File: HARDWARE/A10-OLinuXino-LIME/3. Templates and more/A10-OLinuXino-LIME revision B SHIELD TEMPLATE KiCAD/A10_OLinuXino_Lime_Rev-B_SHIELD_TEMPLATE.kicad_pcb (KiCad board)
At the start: 2 copper layers, 53.2 x 59.6 mm, 5 parts

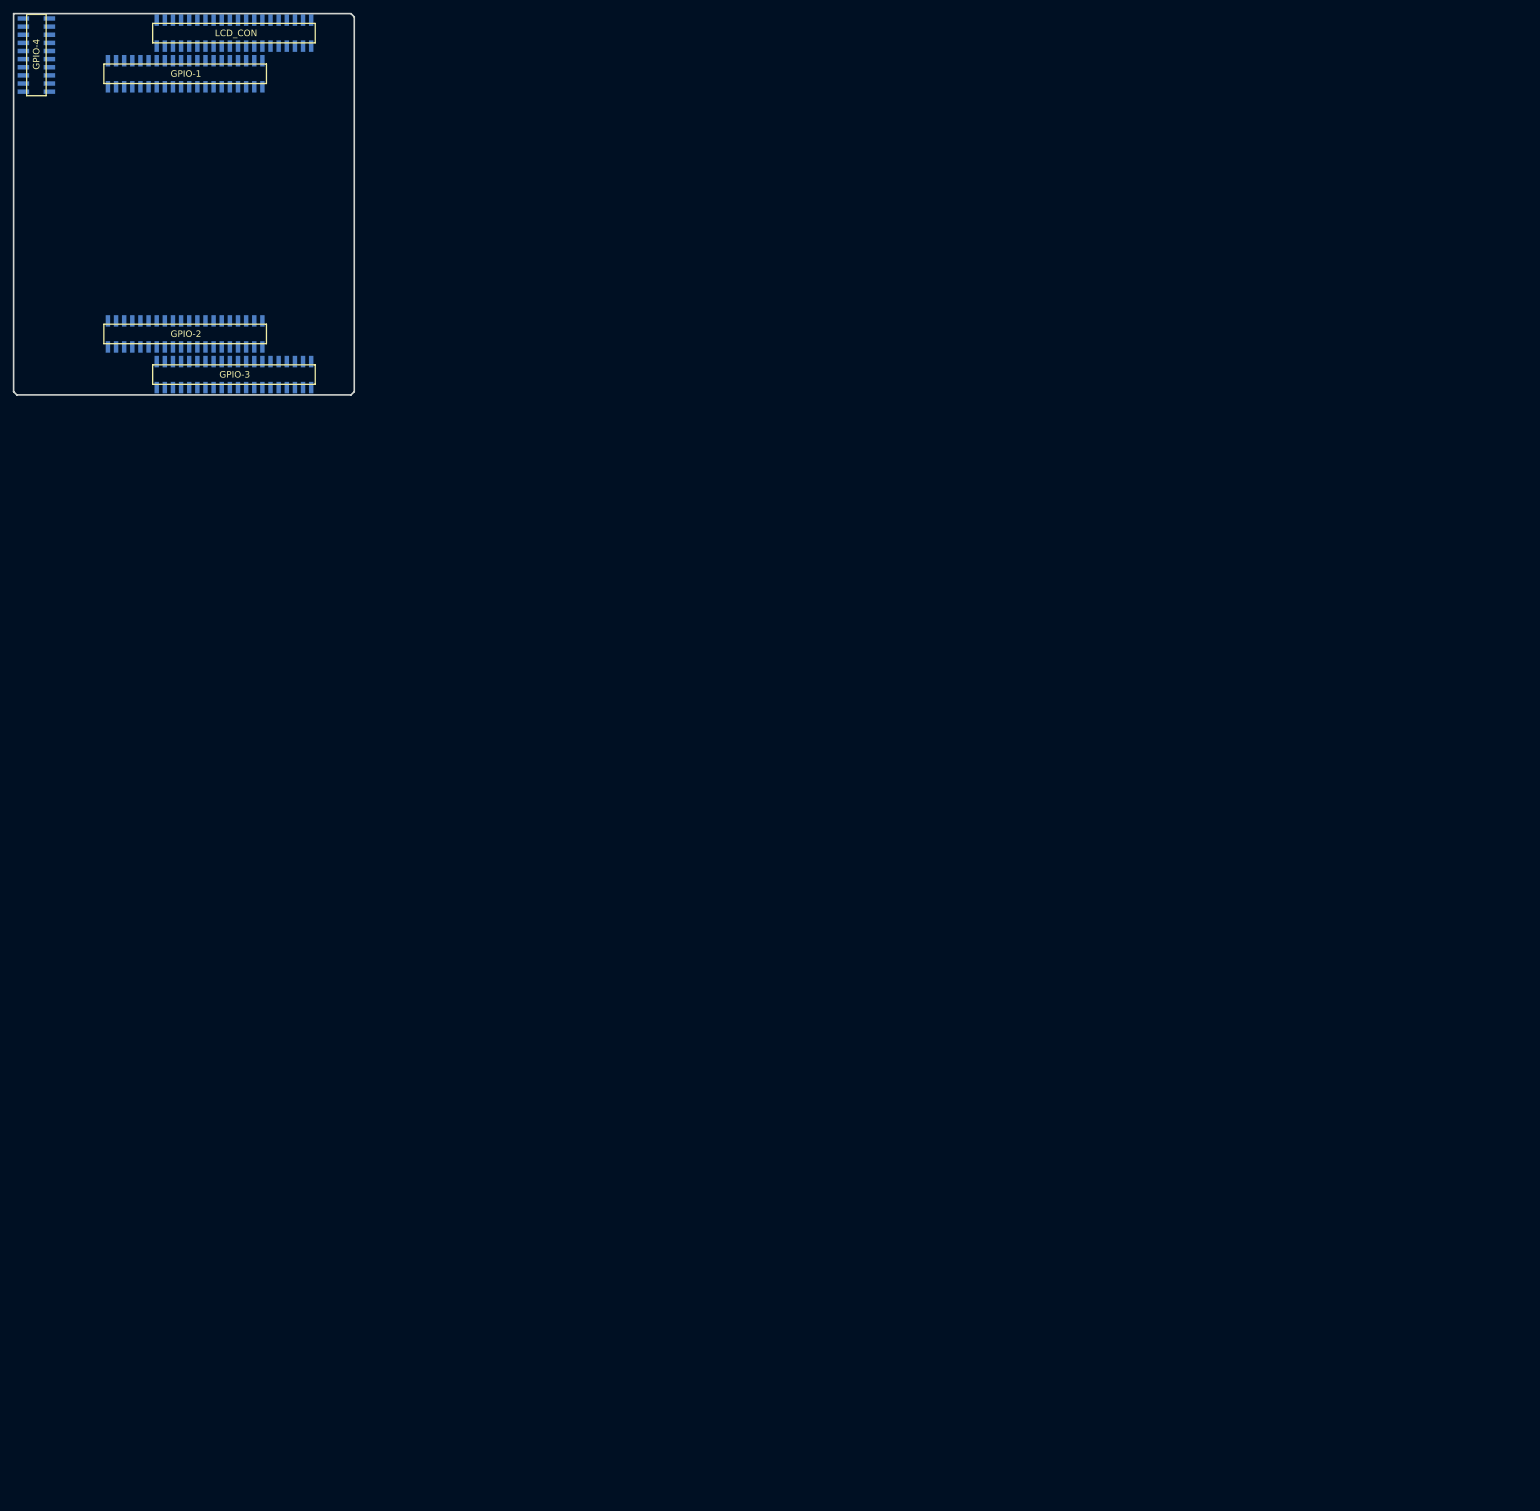
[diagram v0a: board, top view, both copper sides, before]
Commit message: Update
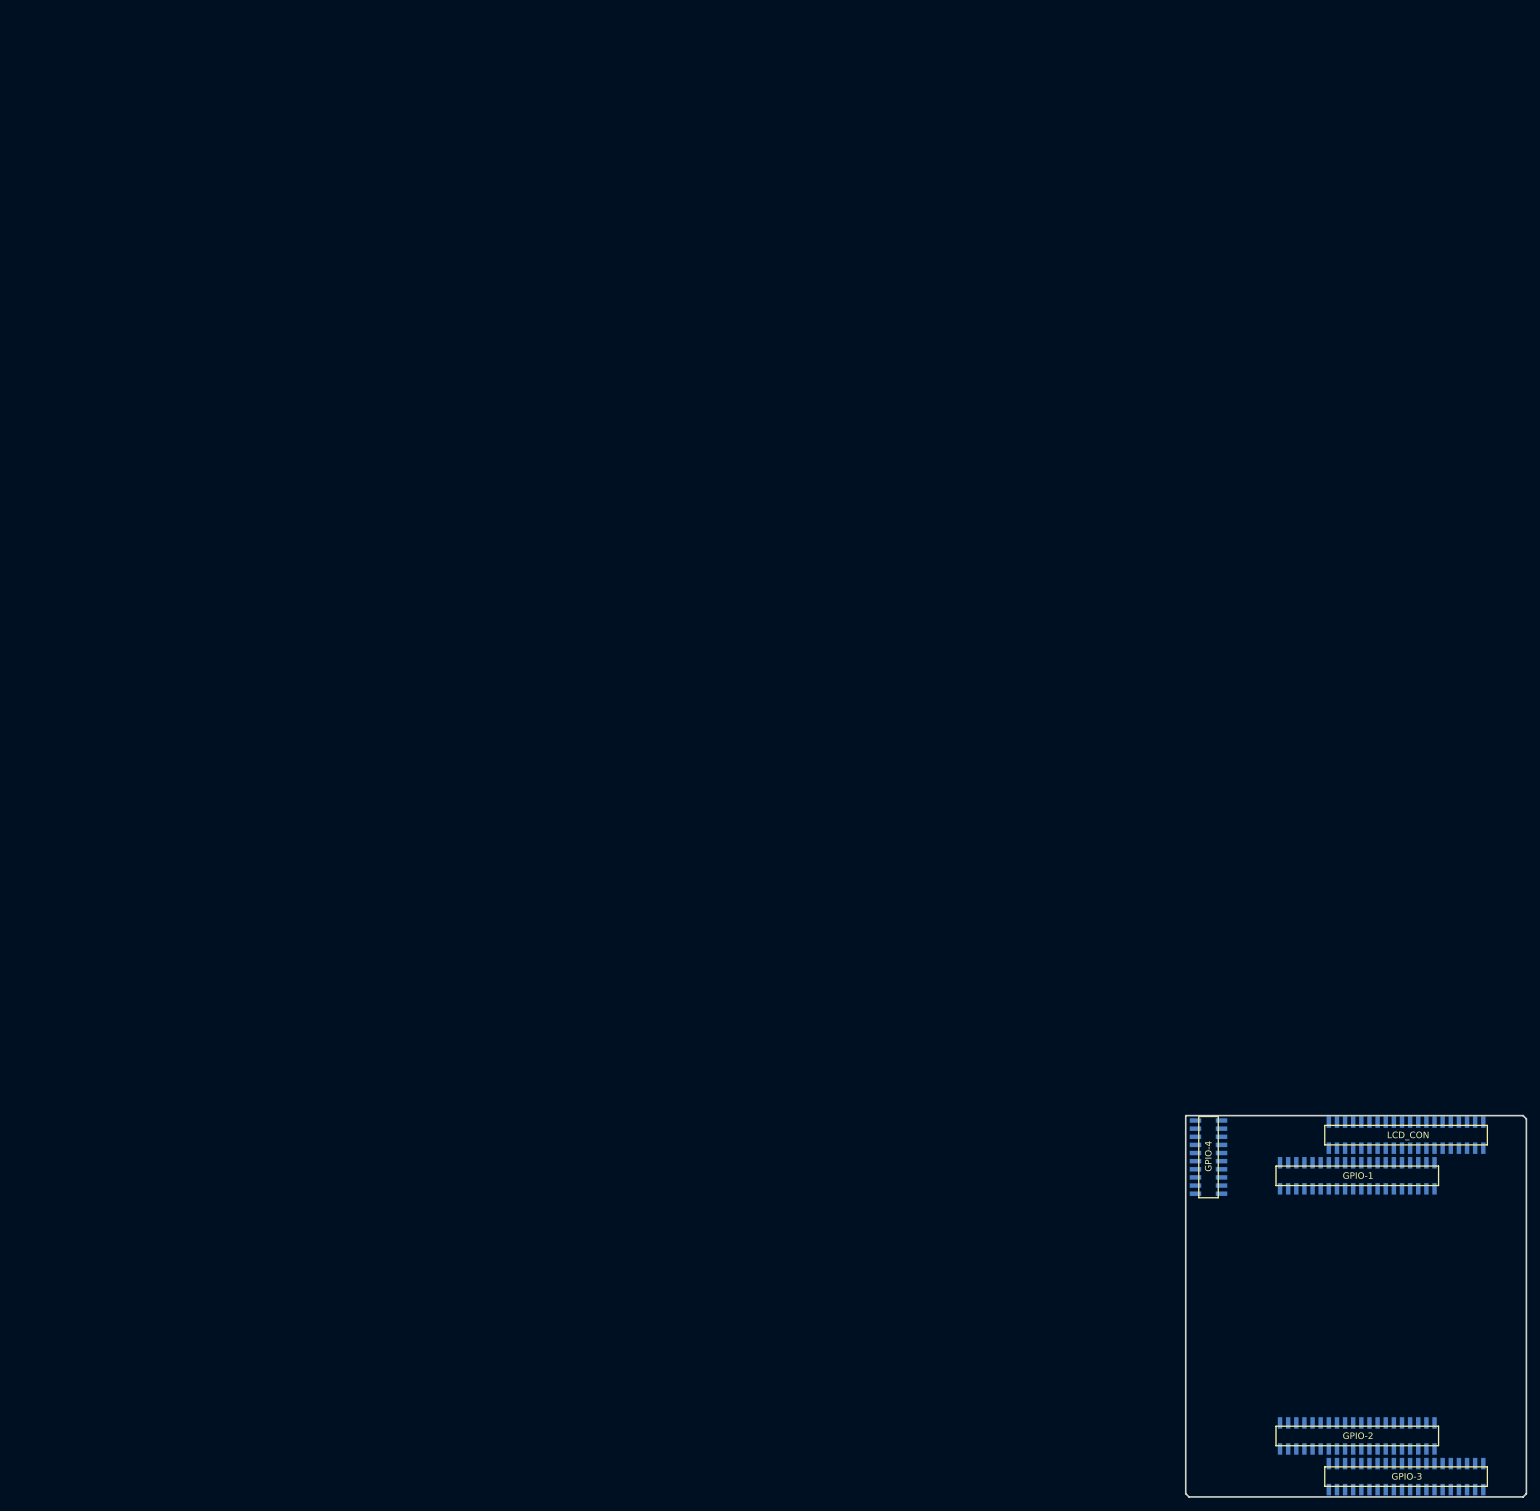
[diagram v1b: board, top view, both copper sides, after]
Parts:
- moved GPIO-1 251.3 mm to (183.3, 151.8)
- moved GPIO-2 251.3 mm to (183.3, 192.4)
- moved LCD_CON1 251.3 mm to (190.9, 145.4)
- moved GPIO-4 251.3 mm to (160.0, 148.8)
- moved GPIO-3 251.3 mm to (190.9, 198.8)
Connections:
- GPIO-1 pad 10: (no net) -> /MICIN1
- GPIO-1 pad 11: (no net) -> /TS1_DVLD/CSI1_VSYNC/SDC1_D1/PG3
- GPIO-1 pad 12: (no net) -> /VMIC
- GPIO-1 pad 13: (no net) -> /TS1_D0/CSI1_D0/SDC1_D2/CSI0_D8/PG4
- GPIO-1 pad 14: (no net) -> /HPOUTL
- GPIO-1 pad 15: (no net) -> /TS1_D1/CSI1_D1/SDC1_D3/CSI0_D9/PG5
- GPIO-1 pad 16: (no net) -> /HPCOM/HPCOMFB
- GPIO-1 pad 17: (no net) -> /TS1_D2/CSI1_D2/UART3_TX/CSI0_D10/PG6
- GPIO-1 pad 18: (no net) -> /HPOUTR
- GPIO-1 pad 19: (no net) -> /TS1_D3/CSI1_D3/UART3_RX/CSI0_D11/PG7
- GPIO-1 pad 20: (no net) -> /TVOUT0/VGA-G
- GPIO-1 pad 21: (no net) -> /TS1_D4/CSI1_D4/UART3_RTS/CSI0_D12/PG8
- GPIO-1 pad 22: (no net) -> /TVOUT1/VGA-B
- GPIO-1 pad 23: (no net) -> /TS1_D5/CSI1_D5/UART3_CTS/CSI0_D13/PG9
- GPIO-1 pad 24: (no net) -> /TVOUT2/VGA-R
- GPIO-1 pad 25: (no net) -> /TS1_D6/CSI1_D6/UART4_TX/CSI0_D14/PG10
- GPIO-1 pad 26: (no net) -> /UART0_RX/IR1_RX/PB23
- GPIO-1 pad 27: (no net) -> /TS1_D7/CSI1_D7/UART4_RX/CSI0_D15/PG11
- GPIO-1 pad 28: (no net) -> /UART0_TX/IR1_TX/PB22
- GPIO-1 pad 29: (no net) -> /NCE1/PC3/SATA-PWR-EN
- GPIO-1 pad 3: +3.3V -> +3V3
- GPIO-1 pad 30: (no net) -> /TWI2_SDA/PB21
- GPIO-1 pad 31: (no net) -> /NCE3/PC18
- GPIO-1 pad 32: (no net) -> /TWI2_SCK/PB20
- GPIO-1 pad 33: (no net) -> /NCE4/SPI2_CS0/PC19
- GPIO-1 pad 34: (no net) -> /TWI1_SDA/PB19
- GPIO-1 pad 35: (no net) -> /NCE5/SPI2_CLK/PC20
- GPIO-1 pad 36: (no net) -> /TWI1_SCK/PB18
- GPIO-1 pad 37: (no net) -> /NCE6/SPI2_MOSI/PC21
- GPIO-1 pad 38: (no net) -> /NDQS/PC24
- GPIO-1 pad 39: (no net) -> /NCE7/SPI2_MISO/PC22
- GPIO-1 pad 4: (no net) -> GNDPWR
- GPIO-1 pad 40: (no net) -> /SPI0_CS0/PC23
- GPIO-1 pad 5: (no net) -> /TS1_CLK/CSI1_PCLK/SDC1_CMD/PG0
- GPIO-1 pad 6: (no net) -> /LRADC0
- GPIO-1 pad 7: (no net) -> /TS1_ERR/CSI1_MLCK/SDC1_CLK/PG1
- GPIO-1 pad 8: (no net) -> /LRADC1
- GPIO-1 pad 9: (no net) -> /TS1_SYNC/CSI1_HSYNC/SDC1_D0/PG2
- GPIO-2 pad 10: (no net) -> /TS0_SYNC/CSI0_HSYNC/PE2
- GPIO-2 pad 11: (no net) -> /GPS_SIGN/PI1
- GPIO-2 pad 12: (no net) -> /TS0_DVLD/CSI0_VSYNC/PE3
- GPIO-2 pad 13: (no net) -> /GPS_MAG/PI2
- GPIO-2 pad 14: (no net) -> /TS0_D0/CSI0_D0/PE4
- GPIO-2 pad 15: (no net) -> /PWM1/PI3
- GPIO-2 pad 16: (no net) -> /TS0_D1/CSI0_D1/PE5
- GPIO-2 pad 17: (no net) -> /SDC3_CMD/PI4
- GPIO-2 pad 18: (no net) -> /TS0_D2/CSI0_D2/PE6
- GPIO-2 pad 19: (no net) -> /SDC3_CLK/PI5
- GPIO-2 pad 20: (no net) -> /TS0_D3/CSI0_D3/PE7
- GPIO-2 pad 21: (no net) -> /SDC3_D0/PI6
- GPIO-2 pad 22: (no net) -> /TS0_D4/CSI0_D4/PE8
- GPIO-2 pad 23: (no net) -> /SDC3_D1/PI7
- GPIO-2 pad 24: (no net) -> /TS0_D5/CSI0_D5/PE9
- GPIO-2 pad 25: (no net) -> /SDC3_D2/PI8
- GPIO-2 pad 26: (no net) -> /TS0_D6/CSI0_D6/PE10
- GPIO-2 pad 27: (no net) -> /SDC3_D3/PI9
- GPIO-2 pad 28: (no net) -> /TS0_D7/CSI0_D7/PE11
- GPIO-2 pad 29: (no net) -> /SPI0_CS0/UART5_TX/EINT22/PI10
- GPIO-2 pad 3: +3.3V -> +3V3
- GPIO-2 pad 30: (no net) -> /HSDA/UART7_RX/PS2_SDA0/PI21
- GPIO-2 pad 31: (no net) -> /SPI0_CLK/UART5_RX/EINT23/PI11
- GPIO-2 pad 32: (no net) -> /HSCL/UART7_TX/PS2_SCK0/PI20
- GPIO-2 pad 33: (no net) -> /SPI0_MOSI/UART6_TX/EINT24/PI12
- GPIO-2 pad 34: (no net) -> /EINT31/SPI1_MISO/UART2_RX/PI19
- GPIO-2 pad 35: (no net) -> /SPI0_MISO/UART6_RX/EINT25/PI13
- GPIO-2 pad 36: (no net) -> /EINT30/SPI1_MOSI/UART2_TX/PI18
- GPIO-2 pad 37: (no net) -> /PS2_SCK1/TCLKIN0/EINT26/SPI0_CS1/PI14
- GPIO-2 pad 38: (no net) -> /EINT29/SPI1_CLK/UART2_CTS/PI17
- GPIO-2 pad 39: (no net) -> /PS2_SDA1/TCLKIN1/EINT27/SPI1_CS1/PI15
- GPIO-2 pad 4: (no net) -> /LDO3_2.8V/VCC_CSI0
- GPIO-2 pad 40: (no net) -> /EINT28/SPI1_CS0/UART2_RTS/PI16
- GPIO-2 pad 5: (no net) -> /TWI0_SCK/PB0
- GPIO-2 pad 6: (no net) -> /TS0_CLK/CSI0_PCLK/PE0
- GPIO-2 pad 7: (no net) -> /TWI0_SDA/PB1
- GPIO-2 pad 8: (no net) -> /TS0_ERR/CSI0_MCLK/PE1
- GPIO-2 pad 9: (no net) -> /GPS_CLK/PI0
- GPIO-3 pad 10: (no net) -> /I2S_MCLK/AC97_MCLK/PB5
- GPIO-3 pad 11: (no net) -> /LCD1_D9/ATAD5/KP_IN1/MS_D1/EINT9/CSI1_D9/PH9
- GPIO-3 pad 12: (no net) -> /I2S_BCLK/AC97_BCLK/PB6
- GPIO-3 pad 13: (no net) -> /LCD1_D10/ATAD6/KP_IN2/MS_D2/EINT10/CSI1_D10/PH10
- GPIO-3 pad 14: (no net) -> /I2S_LRCK/AC97_SYNC/PB7
- GPIO-3 pad 15: (no net) -> /LCD1_D11/ATAD7/KP_IN3/MS_D3/EINT11/CSI1_D11/PH11
- GPIO-3 pad 16: (no net) -> /I2S_DO0/AC97_DO/PB8/SATA-PWR-EN
- GPIO-3 pad 17: (no net) -> /LCD1_D12/ATAD8/PS2_SCK1/EINT12/CSI1_D12/PH12
- GPIO-3 pad 18: (no net) -> /I2S_DO2/PB10
- GPIO-3 pad 19: (no net) -> /LCD1_D13/ATAD9/PS2_SDA1/SMC_RST/EINT13/CSI1_D13/PH13
- GPIO-3 pad 20: (no net) -> /I2S_DO3/PB11
- GPIO-3 pad 21: (no net) -> /LCD1_D14/ATAD10/KP_IN4/SMC_VPPEN/EINT14/CSI1_D14/PH14
- GPIO-3 pad 22: (no net) -> /I2S_DI/AC97_DI/SPDIF_DI/PB12
- GPIO-3 pad 23: (no net) -> /LCD1_D15/ATAD11/KP_IN5/SMC_VPPPP/EINT15/CSI1_D15/PH15
- GPIO-3 pad 24: (no net) -> /SPI2_CS1/SPDIF_DO/PB13
- GPIO-3 pad 25: (no net) -> /LCD1_D16/ATAD12/KP_IN6/SMC_DET/EINT16/CSI1_D16/PH16
- GPIO-3 pad 26: (no net) -> /JTAG_MS0/SPI2_CS0/PB14
- GPIO-3 pad 27: (no net) -> /LCD1_D17/ATAD13/KP_IN7/SMC_VCCEN/EINT17/CSI1_D17/PH17
- GPIO-3 pad 28: (no net) -> /JTAG_CK0/SPI2_CLK/PB15
- GPIO-3 pad 29: (no net) -> /LCD1_D18/ATAD14/KP_OUT0/SMC_SLK/EINT18/CSI1_D18/PH18
- GPIO-3 pad 3: (no net) -> +3V3
- GPIO-3 pad 30: (no net) -> /JTAG_DO0/SPI2_MOSI/PB16
- GPIO-3 pad 31: (no net) -> /LCD1_D19/ATAD15/KP_OUT1/SMC_SDA/EINT19/CSI1_D19/PH19
- GPIO-3 pad 32: (no net) -> /JTAG_DI0/SPI2_MISO/PB17
- GPIO-3 pad 33: (no net) -> /LCD1_D20/ATAOE/CAN_TX/EINT20/CSI1_D20/PH20
- GPIO-3 pad 34: (no net) -> /LCD1_CLK/ATACS1/KP_OUT4/SDC1_D0/CSI1_PCLK/PH24
- GPIO-3 pad 35: (no net) -> /LCD1_D21/ATADREQ/CAN_RX/EINT21/CSI1_D21/PH21
- GPIO-3 pad 36: (no net) -> /LCD1_DE/ATAIORDY/KP_OUT5/SDC1_D1/CSI1_FIELD/PH25
- GPIO-3 pad 37: (no net) -> /LCD1_D22/ATADACK/KP_OUT2/SDC1_CMD/CSI1_D22/PH22
- GPIO-3 pad 38: (no net) -> /LCD1_HSYNC/ATAIOR/KP_OUT6/SDC1_D2/CSI1_HSYNC/PH26
- GPIO-3 pad 39: (no net) -> /LCD1_D23/ATACS0/KP_OUT3/SDC1_CLK/CSI1_D23/PH23
- GPIO-3 pad 40: (no net) -> /LCD1_VSYNC/ATAIOW/KP_OUT7/SDC1_D3/CSI1_VSYNC/PH27
- GPIO-3 pad 5: (no net) -> /RESET_N
- GPIO-3 pad 6: (no net) -> /IR0_TX/SPDIF_MCLK/STANBYWFI/PB3
- GPIO-3 pad 7: (no net) -> /LCD1_D0/ATAA0/UART3_TX/EINT0/CSI1_D0/PH0
- GPIO-3 pad 8: (no net) -> /IR0_RX/PB4
- GPIO-3 pad 9: (no net) -> /LCD1_D7/ATAD3/UART5_RX/MS_CLK/EINT7/CSI1_D7/PH7/I2S_DO1/PB9/USB0-DRV
- GPIO-4 pad 1: +3.3V -> +3V3
- GPIO-4 pad 10: (no net) -> /MICIN2
- GPIO-4 pad 11: (no net) -> /TVIN3
- GPIO-4 pad 12: (no net) -> /GPIO2
- GPIO-4 pad 13: (no net) -> /LINEINR
- GPIO-4 pad 14: (no net) -> /GPIO3
- GPIO-4 pad 15: (no net) -> /LINEINL
- GPIO-4 pad 16: (no net) -> /NRB1/SDC2_CLK/PC7
- GPIO-4 pad 17: (no net) -> /FMINR
- GPIO-4 pad 18: (no net) -> /NWP/PC16
- GPIO-4 pad 19: (no net) -> /FMINL
- GPIO-4 pad 20: (no net) -> /NCE2/PC17
- GPIO-4 pad 3: (no net) -> /TVOUT3
- GPIO-4 pad 4: (no net) -> /NMI_N
- GPIO-4 pad 5: (no net) -> /TVIN0
- GPIO-4 pad 6: (no net) -> /MIC1OUTP
- GPIO-4 pad 7: (no net) -> /TVIN1
- GPIO-4 pad 8: (no net) -> /MIC1OUTN
- GPIO-4 pad 9: (no net) -> /TVIN2
- LCD_CON1 pad 10: (no net) -> /LCD0_D21/SMC_VPPEN/PD21
- LCD_CON1 pad 11: (no net) -> /LCD0_D22/SMC_VPPPP/PD22
- LCD_CON1 pad 12: (no net) -> /LCD0_D23/SMC_DET/PD23
- LCD_CON1 pad 13: (no net) -> /LCD0_D8/LVDS0_VP3/PD8
- LCD_CON1 pad 14: (no net) -> /LCD0_D9/LVDS0_VN3/PD9
- LCD_CON1 pad 15: (no net) -> /LCD0_D10/LVDS1_VP0/PD10
- LCD_CON1 pad 16: (no net) -> /LCD0_D11/LVDS1_VN0/PD11
- LCD_CON1 pad 17: (no net) -> /LCD0_D12/LVDS1_VP1/PD12
- LCD_CON1 pad 18: (no net) -> /LCD0_D13/LVDS1_VN1/PD13
- LCD_CON1 pad 19: (no net) -> /LCD0_D14/LVDS1_VP2/PD14
- LCD_CON1 pad 20: (no net) -> /LCD0_D15/LVDS1_VN2/PD15
- LCD_CON1 pad 21: (no net) -> /LCD0_D0/LVDS0_VP0/PD0
- LCD_CON1 pad 22: (no net) -> /LCD0_D1/LVDS0_VN0/PD1
- LCD_CON1 pad 23: (no net) -> /LCD0_D2/LVDS0_VP1/PD2
- LCD_CON1 pad 24: (no net) -> /LCD0_D3/LVDS0_VN1/PD3
- LCD_CON1 pad 25: (no net) -> /LCD0_D4/LVDS0_VP2/PD4
- LCD_CON1 pad 26: (no net) -> /LCD0_D5/LVDS0_VN2/PD5
- LCD_CON1 pad 27: (no net) -> /LCD0_D6/LVDS0_VPC/PD6
- LCD_CON1 pad 28: (no net) -> /LCD0_D7/LVDS0_VNC/PD7
- LCD_CON1 pad 29: (no net) -> /LCD0_HSYNC/SMC_SLK/PD26
- LCD_CON1 pad 3: +3.3V -> +3V3
- LCD_CON1 pad 30: (no net) -> /LCD0_VSYNC/SMC_SDA/PD27
- LCD_CON1 pad 31: (no net) -> /LCD0_CLK/SMC_VCCEN/PD24
- LCD_CON1 pad 32: (no net) -> /LCD0_DE/SMC_RST/PD25
- LCD_CON1 pad 33: (no net) -> /NC/IR0_TX/SPDIF_MCLK/STANBYWFI/PB3
- LCD_CON1 pad 34: (no net) -> /NC/IR0_RX/PB4
- LCD_CON1 pad 35: (no net) -> /LCD1_D8/ATAD4/KP_IN0/MS_D0/EINT8/CSI1_D8/PH8
- LCD_CON1 pad 36: (no net) -> /PB2/PWM0
- LCD_CON1 pad 37: (no net) -> /XP_TP
- LCD_CON1 pad 38: (no net) -> /XN_TP
- LCD_CON1 pad 39: (no net) -> /YP_TP
- LCD_CON1 pad 40: (no net) -> /YN_TP
- LCD_CON1 pad 5: (no net) -> /LCD0_D16/LVDS1_VPC/PD16
- LCD_CON1 pad 6: (no net) -> /LCD0_D17/LVDS1_VNC/PD17
- LCD_CON1 pad 7: (no net) -> /LCD0_D18/LVDS1_VP3/PD18
- LCD_CON1 pad 8: (no net) -> /LCD0_D19/LVDS1_VN3/PD19
- LCD_CON1 pad 9: (no net) -> /LCD0_D20/CSI1_MCLK/PD20
